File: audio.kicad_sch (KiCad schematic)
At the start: 6 parts, among them J1 USB4105-GF-A, U1 PCM5102APW, U2 TPA6130A2RTJR, U3 DEV-15583

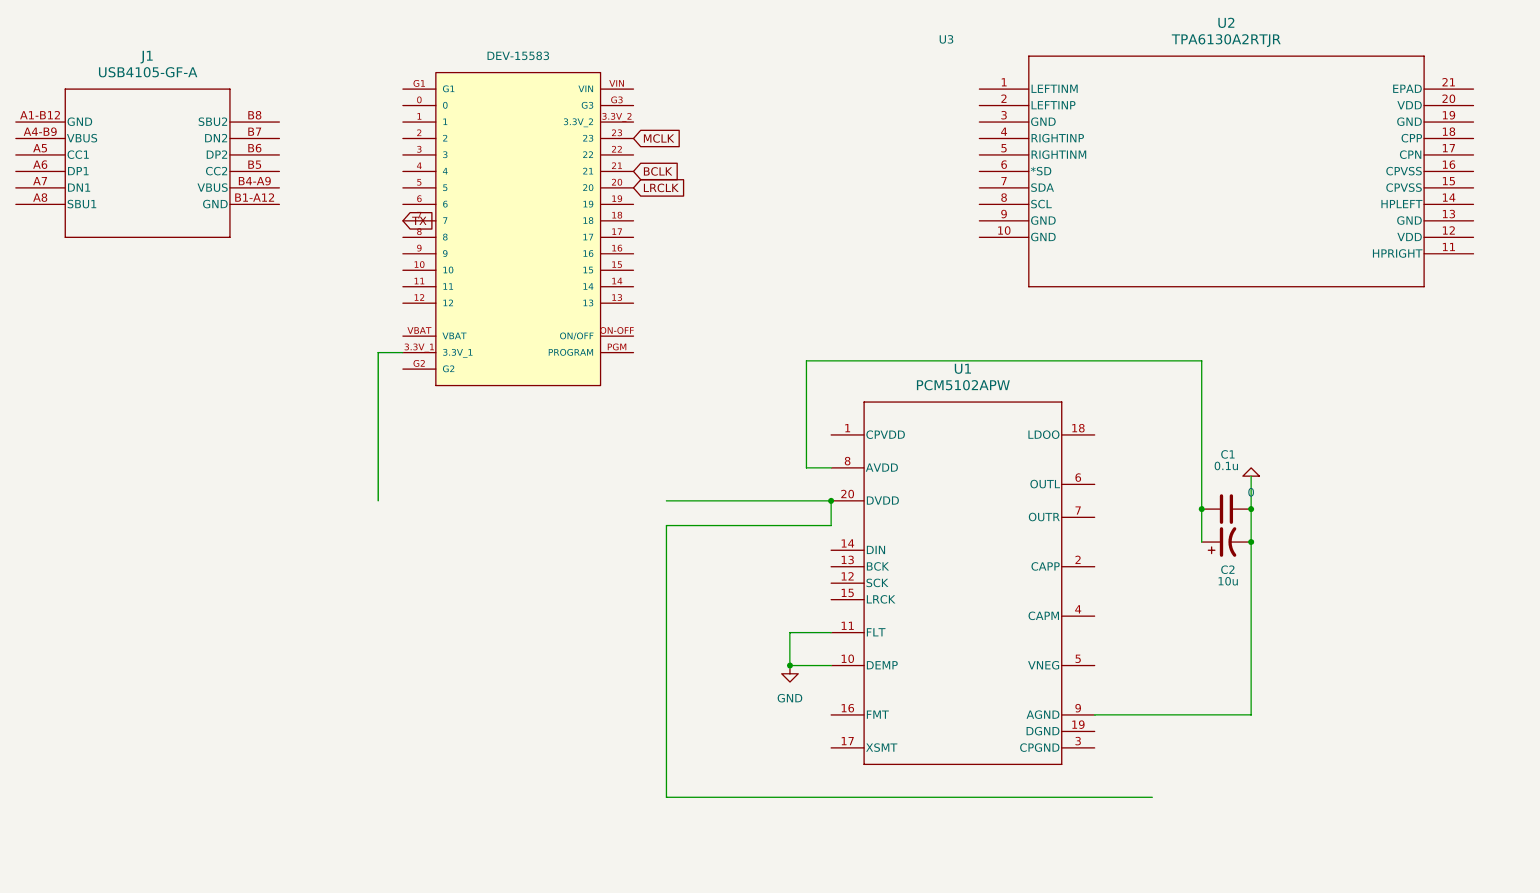
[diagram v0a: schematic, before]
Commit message: vähän lisää piirtelin
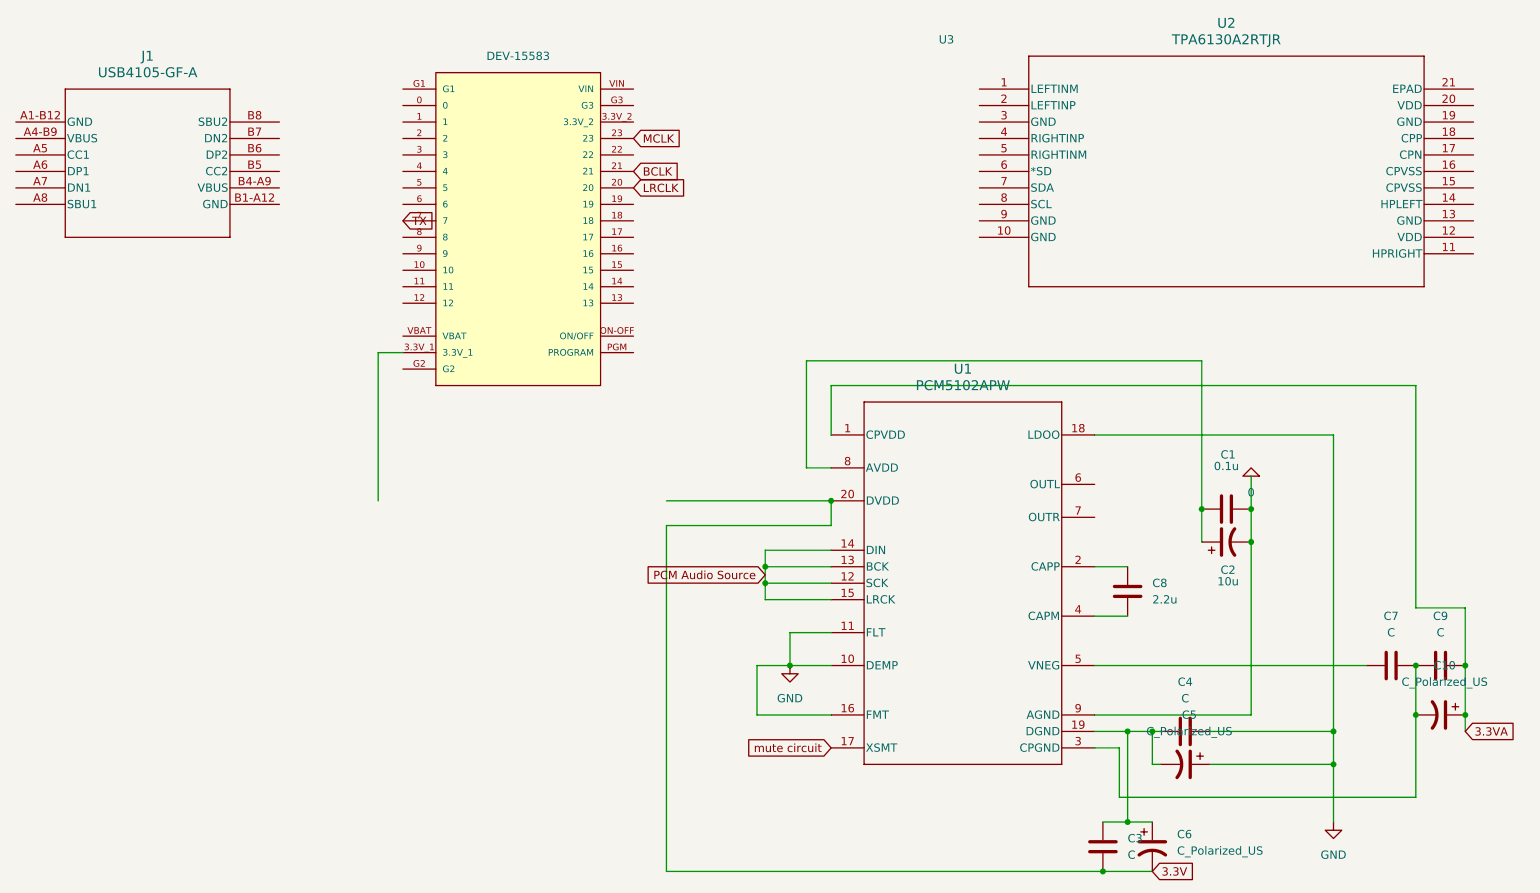
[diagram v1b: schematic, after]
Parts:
- added C10, C5, C6: C_Polarized_US, symbol Device:C_Polarized_US
- added C3, C4, C7, C9: C, symbol Device:C
- added C8: 2.2u, symbol Device:C
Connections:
- net GND: now also U1.16 (FMT), U1.18 (LDOO), C4.2, C5.1
- net 3.3VA: now reaches U1.1 (CPVDD)
- net 3.3VA: now also C10.1, C9.2
- net PCM Audio Source: now reaches U1.12 (SCK)
- net PCM Audio Source: now also U1.13 (BCK), U1.14 (DIN), U1.15 (LRCK)
- net mute circuit: now reaches U1.17 (XSMT)
- net at U1.19 (DGND): now also C3.1, C4.1, C5.2, C6.1
- net at U1.2 (CAPP): now also C8.1
- net 3.3V: now reaches U1.20 (DVDD)
- net 3.3V: now also C3.2, C6.2
- net at U1.3 (CPGND): now also C10.2, C7.2, C9.1
- net at U1.4 (CAPM): now also C8.2
- net at U1.5 (VNEG): now also C7.1
